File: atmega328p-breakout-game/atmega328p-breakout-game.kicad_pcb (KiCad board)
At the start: 2 copper layers, 68 x 58.4 mm, 28 parts, among them J1 Conn_Battery 4.5V, Q1 DTC113Z, Q2 DTC113Z, Q3 DTC113Z, Q4 DTC113Z, Q5 DTC113Z, Q6 DTC113Z, Q7 DTC113Z, Q8 DTC113Z, SW1 SW_RESET, SW2 SW_MOVE_RIGHT, SW3 SW_MOVE_LEFT, SW4 SW_DPDT_x2, U1 ATmega328P-P, U2 D15881-M-UR3-0-W

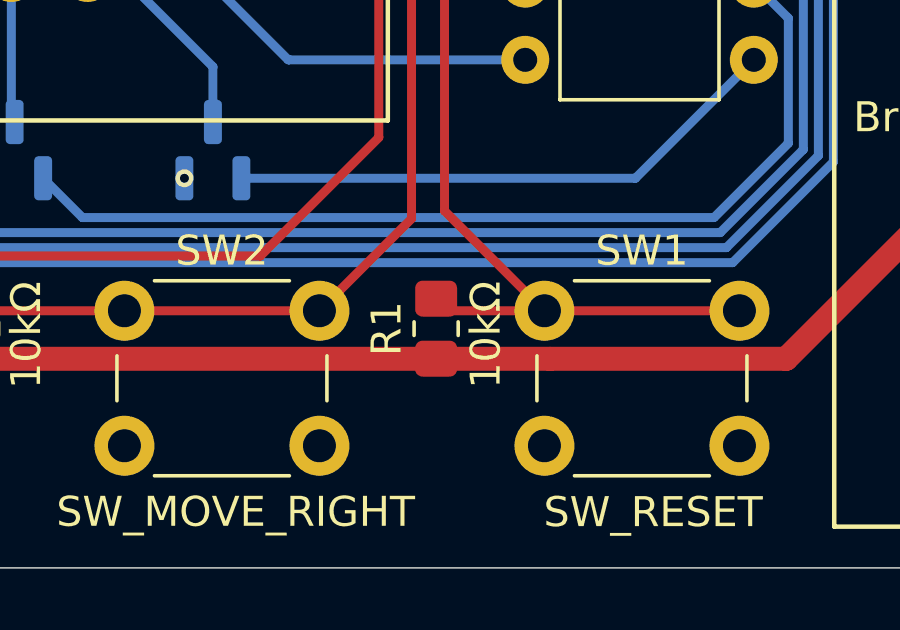
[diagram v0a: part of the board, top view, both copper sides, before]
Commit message: a
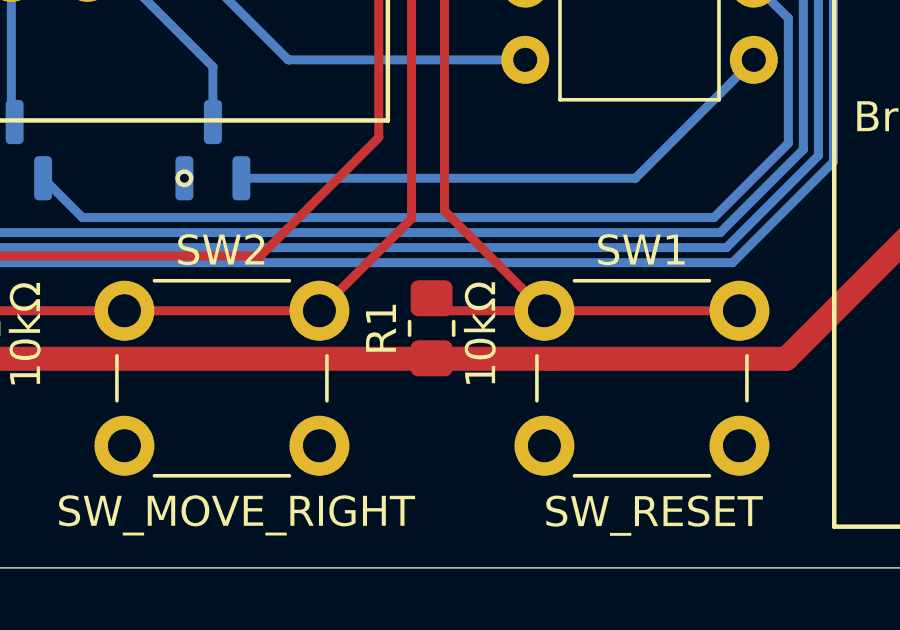
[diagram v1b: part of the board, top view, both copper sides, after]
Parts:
- moved R1 0.15 mm to (160.3, 112.2)
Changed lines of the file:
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@@
 	(footprint "Resistor_SMD:R_0805_2012Metric_Pad1.20x1.40mm_HandSolder"
 		(layer "F.Cu")
-		(at 160.41 112.24 90)
+		(at 160.26 112.23 90)
 		(descr "Resistor SMD 0805 (2012 Metric), square (rectangular) end terminal, IPC-7351 nominal with elongated pad for handsoldering. (Body size source: IPC-SM-782 page 72, https://www.pcb-3d.com/wordpress/wp-content/uploads/ipc-sm-782a_amendment_1_and_2.pdf), generated with kicad-footprint-generator")
 		(tags "resistor handsolder")
@@
 	)
 	(gr_text "10kΩ"
-		(at 162.65 114.24 90)
+		(at 162.5 114.23 90)
 		(layer "F.SilkS")
 		(effects
@@
 	)
 	(segment
-		(start 160.813737 111.643737)
-		(end 160.41 111.24)
+		(start 162.68 70.26)
+		(end 160.69 72.25)
 		(width 0.3)
 		(layer "F.Cu")
@@
 	)
 	(segment
-		(start 162.68 70.26)
-		(end 160.69 72.25)
+		(start 160.69 72.25)
+		(end 160.69 108.313737)
 		(width 0.3)
 		(layer "F.Cu")
@@
 	)
 	(segment
-		(start 160.69 72.25)
-		(end 160.69 108.313737)
+		(start 160.673737 111.643737)
+		(end 160.26 111.23)
 		(width 0.3)
 		(layer "F.Cu")
@@
 	(segment
 		(start 164.02 111.643737)
-		(end 160.813737 111.643737)
+		(end 160.673737 111.643737)
 		(width 0.3)
 		(layer "F.Cu")
